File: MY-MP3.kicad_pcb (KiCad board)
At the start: 4 copper layers, 37 x 90 mm, 86 parts, among them J1 microSD, J2 USB_C_Receptacle, J3 JST_2mm_LiPo, J4 Adafruit 5393 Headers, J7 AudioJack3_SwitchTR, J9 Conn_01x04_FPC, Q1 DMG3415U, SW1 SMD_6x3.5mm_h2.5mm, SW2 SMD_6x3.5mm_h2.5mm, SW3 BTN_POW, SW4 BTN_VUP, SW5 BTN_VDN, SW6 Nav Switch, SW7 BTN_OPT, SW8 BTN_SEL, U1 STM32L4R5VITx, U2 CODECODER-VS1053B_LQFP48_, U3 RT9080-3.3, U4 MAX17048, U5 STM6601, U6 MCP73831-2-OT, U7 AP7312-1833W6, Y1 ABM3-12.288MHZ-D2Y-T, Y2 8 mHz

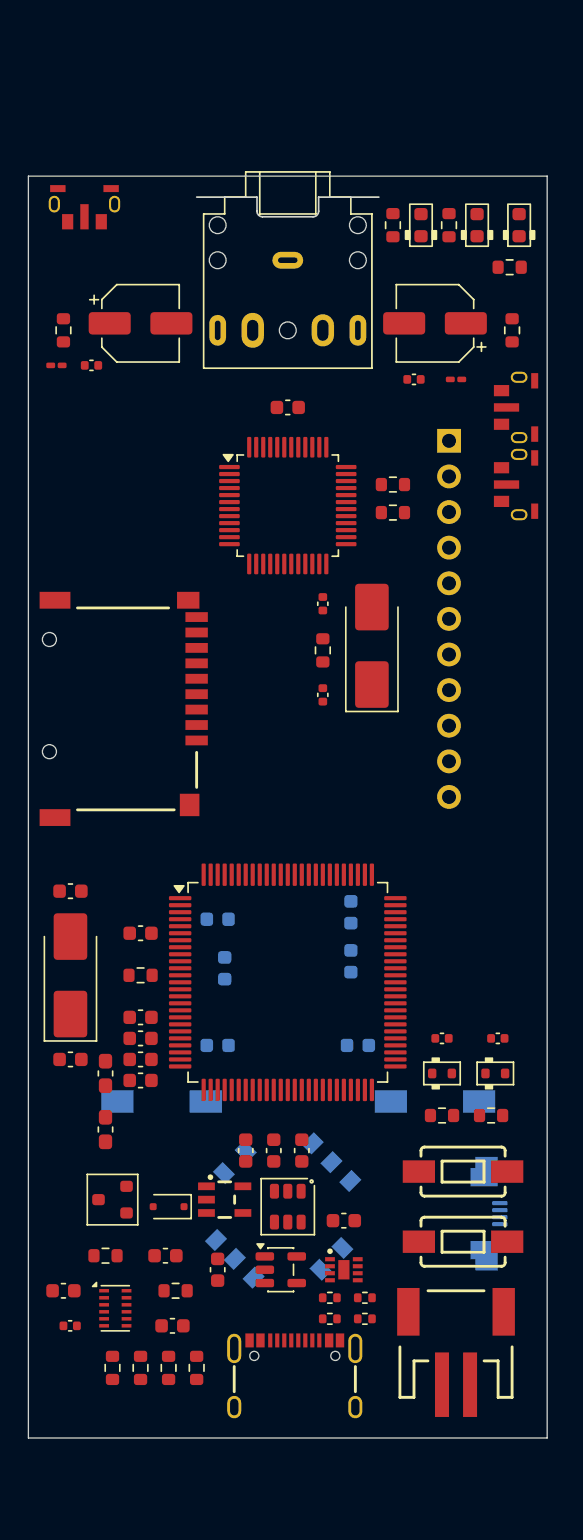
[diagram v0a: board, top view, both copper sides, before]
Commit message: Finish PCB
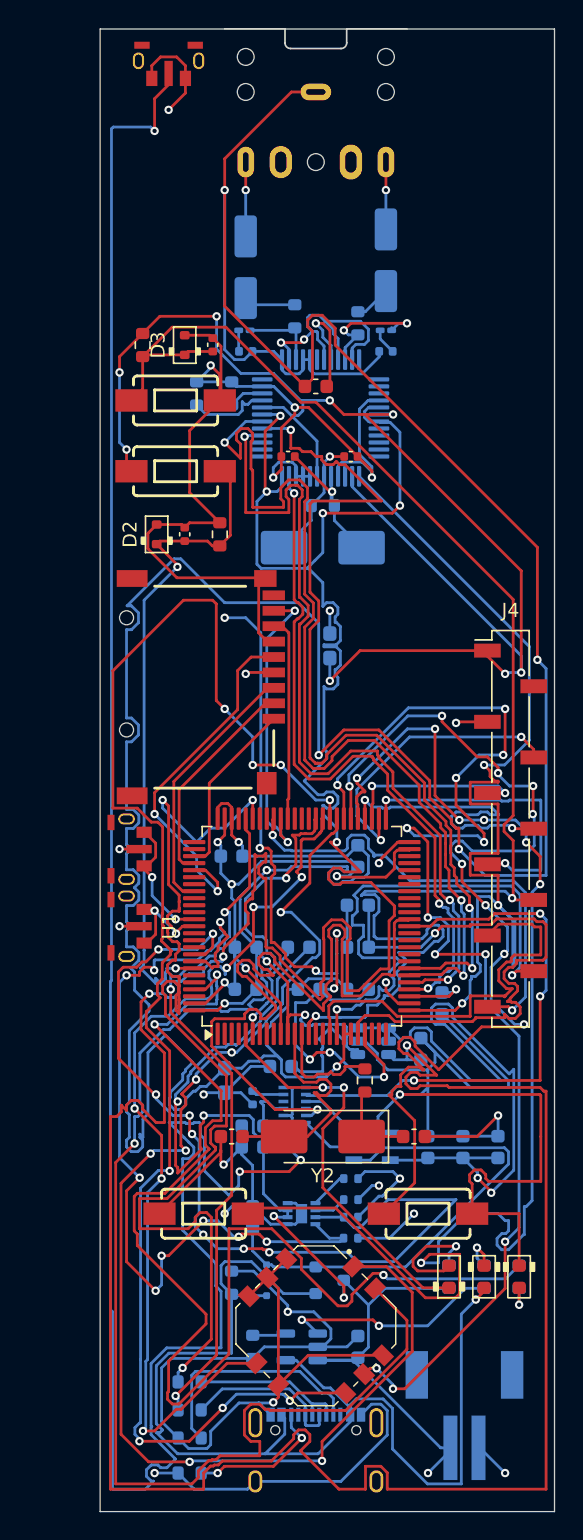
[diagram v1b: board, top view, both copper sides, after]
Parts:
- removed J9: Conn_01x04_FPC, Connector_FFC-FPC:Amphenol_F32Q-1A7x1-11004_1x04-1MP_P0.5mm_Horizontal
- C1, C10, C14, C16, C2, C22, C23, C25, C26, C27, C28, C29, C3, C30, C31, C7, C8, C9, D1, FB1, FB2, J2, J3, J7, Q1, R1, R10, R12, R13, R14, R15, R16, R18, R19, R2, R20, R22, R23, R25, R4, R5, R6, R7, R8, R9, U2, U3, U4, U5, U6, U7, Y1: moved to B.Cu
- J4: footprint Connector_PinSocket_2.54mm:PinSocket_1x11_P2.54mm_Vertical -> Connector_PinSocket_2.54mm:PinSocket_1x11_P2.54mm_Vertical_SMD_Pin1Left; moved to F.Cu
- SW6, SW7, SW8: moved to F.Cu
- moved R25 75.5 mm to (174.5, 126.5), turned to 90 degrees
- moved LED2 75.3 mm to (174.5, 126.5), turned to -90 degrees
- moved LED3 75.2 mm to (169.5, 126.5)
- moved R20 75.0 mm to (172.0, 126.5), turned to -90 degrees
- moved LED1 75.0 mm to (172.0, 126.5), turned to -90 degrees
- moved R16 72.1 mm to (169.5, 126.5), turned to -90 degrees
- moved R21 59.0 mm to (147.7, 60.0), turned to -90 degrees
- moved SW1 58.7 mm to (150.0, 64.0)
- moved SW2 58.6 mm to (150.0, 69.0)
- moved D3 55.1 mm to (150.7, 60.0), turned to 90 degrees
- moved C15 52.1 mm to (152.7, 60.0), turned to 90 degrees
- moved R3 45.7 mm to (153.2, 73.5), turned to 90 degrees
- moved D2 45.4 mm to (148.7, 73.5), turned to 90 degrees
- moved C24 42.3 mm to (150.7, 73.5), turned to 90 degrees
- moved SW4 42.1 mm to (146.5, 96.0), turned to 90 degrees
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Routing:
- net GND: track 0.00 -> 344.7 mm, vias 0 -> 24
- net 1.8V: track 0.00 -> 260.8 mm, vias 0 -> 8
- net GNDA: track 0.00 -> 254.5 mm, vias 0 -> 5
- net 3.3V: track 0.00 -> 192.6 mm, vias 0 -> 18
- net Net-(U5-~{PB}): track 0.00 -> 165.4 mm, vias 0 -> 3
- net /BTN_DN: track 0.00 -> 108.0 mm, vias 0 -> 8
- net /NRST: track 0.00 -> 104.6 mm, vias 0 -> 2
- net /BTN_SEEK: track 0.00 -> 96.8 mm, vias 0 -> 2
- net /BTN_UP: track 0.00 -> 90.7 mm, vias 0 -> 7
- net /BTN_PLAY: track 0.00 -> 90.1 mm, vias 0 -> 12
- net /BTN_OPT: track 0.00 -> 90.0 mm, vias 0 -> 7
- net /LED: track 0.00 -> 85.8 mm, vias 0 -> 3
- net VBATT: track 0.00 -> 82.5 mm, vias 0 -> 5
- net VBUS: track 0.00 -> 81.5 mm, vias 0 -> 1
- net 3.3V_A: track 0.00 -> 80.9 mm, vias 0 -> 11
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- added copper zone on In1.Cu, net 3.3V_A
- added copper zone on In1.Cu, net VBATT
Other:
- board size 37 x 90 mm -> 32.4 x 105.7 mm
- board text removed: "LED1"
